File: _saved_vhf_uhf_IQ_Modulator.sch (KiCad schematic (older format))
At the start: 60 parts

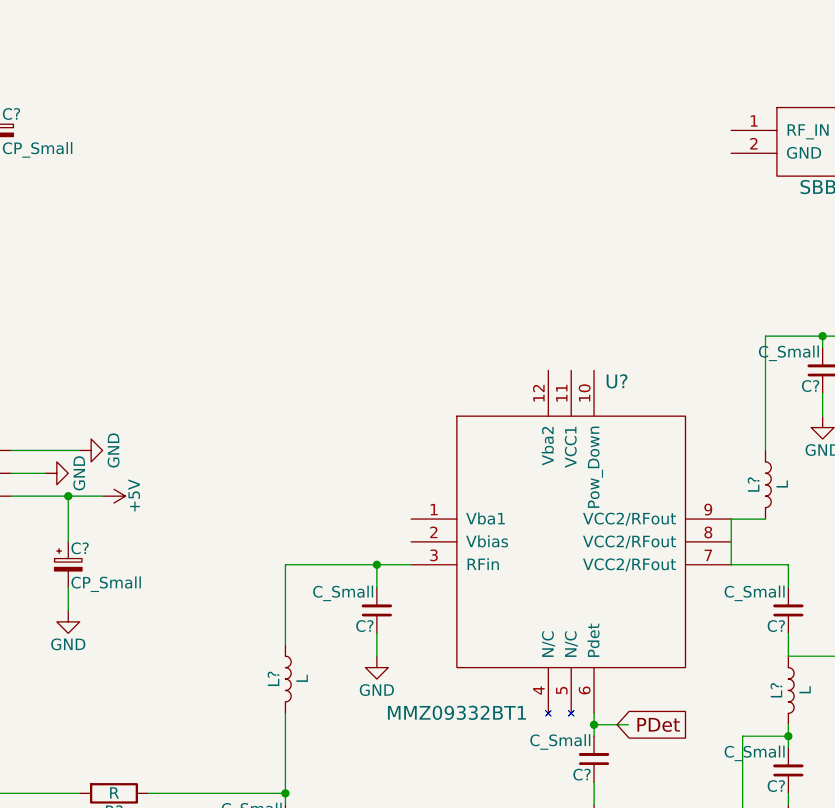
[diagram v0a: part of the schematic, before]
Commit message: added dokumets
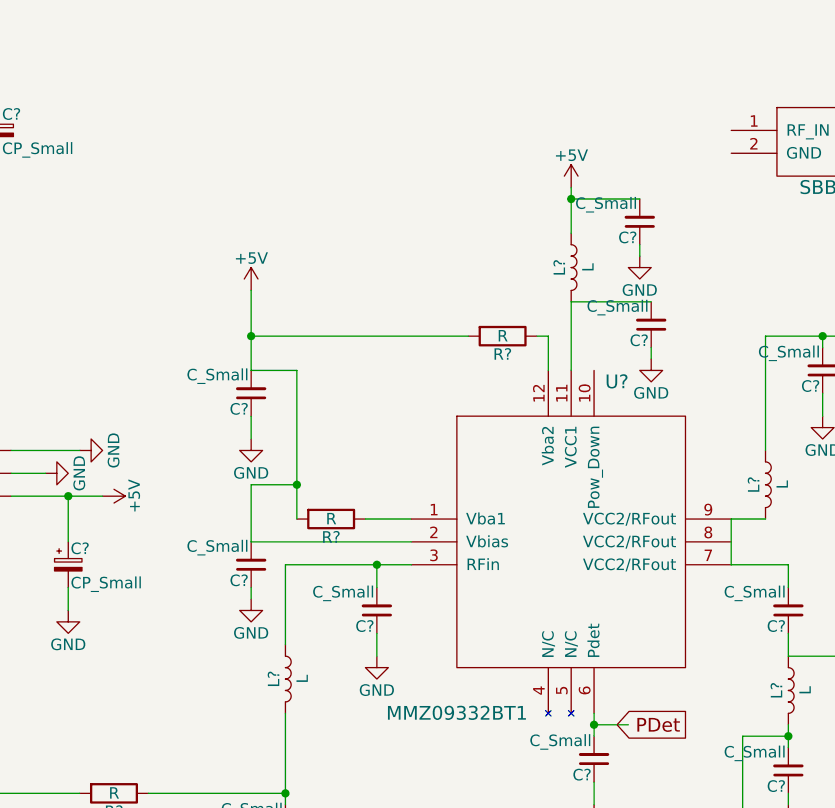
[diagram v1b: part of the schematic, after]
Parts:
- removed U?: MMZ09332BT1, symbol MMZ09332BT1
- added C? (x4): C_Small, symbol C_Small
- added L?: L, symbol L
- added R? (x2): R, symbol R
- added U?: MMZ09332BT1, symbol MMZ09332BT1
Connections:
- net +5V: now also C?.2, C?.2, C?.2, L?.1, R?.2, R?.2, U?.2 (Vbias)
- net GND: now also C?.1, C?.1, C?.1, C?.1
- net at C?.2, L?.1: now also U?.3 (RFin)
- net at C?.2: now also U?.6 (Pdet)
- net at C?.2, L?.2: now also U?.7 (VCC2/RFout), U?.9 (VCC2/RFout)
- new net: C?.2, L?.2, U?.11 (VCC1)
- new net: R?.1, U?.1 (Vba1)
- new net: R?.1, U?.12 (Vba2)
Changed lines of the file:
@@
-$EndComp
-$Comp
-L MMZ09332BT1 U?
-U 1 1 5A2315D3
-P 12850 3000
-F 0 "U?" H 13050 3700 60  0000 C CNN
-F 1 "MMZ09332BT1" H 12350 2250 60  0000 C CNN
-F 2 "" H 12850 3000 60  0001 C CNN
-F 3 "" H 12850 3000 60  0001 C CNN
-	1    12850 3000
-	1    0    0    -1
 $EndComp
 $Comp
@@
 	13100 3800 12950 3800
 Connection ~ 12950 3800
+$Comp
+L L L?
+U 1 1 5A2373B0
+P 12850 1800
+F 0 "L?" V 12800 1800 50  0000 C CNN
+F 1 "L" V 12925 1800 50  0000 C CNN
+F 2 "" H 12850 1800 50  0001 C CNN
+F 3 "" H 12850 1800 50  0001 C CNN
+	1    12850 1800
+	1    0    0    -1
+$EndComp
+$Comp
+L C_Small C?
+U 1 1 5A2374AB
+P 13200 2050
+F 0 "C?" H 13210 2120 50  0000 L CNN
+F 1 "C_Small" H 13210 1970 50  0000 L CNN
+F 2 "" H 13200 2050 50  0001 C CNN
+F 3 "" H 13200 2050 50  0001 C CNN
+	1    13200 2050
+	-1   0    0    1
+$EndComp
+$Comp
+L C_Small C?
+U 1 1 5A237595
+P 13150 1600
+F 0 "C?" H 13160 1670 50  0000 L CNN
+F 1 "C_Small" H 13160 1520 50  0000 L CNN
+F 2 "" H 13150 1600 50  0001 C CNN
+F 3 "" H 13150 1600 50  0001 C CNN
+	1    13150 1600
+	-1   0    0    1
+$EndComp
+Wire Wire Line
+	12850 2250 12850 1950
+Wire Wire Line
+	12850 1950 13200 1950
+$Comp
+L GND #PWR?
+U 1 1 5A237928
+P 13200 2200
+F 0 "#PWR?" H 13200 1950 50  0001 C CNN
+F 1 "GND" H 13200 2050 50  0000 C CNN
+F 2 "" H 13200 2200 50  0001 C CNN
+F 3 "" H 13200 2200 50  0001 C CNN
+	1    13200 2200
+	1    0    0    -1
+$EndComp
+$Comp
+L GND #PWR?
+U 1 1 5A237A2F
+P 13150 1750
+F 0 "#PWR?" H 13150 1500 50  0001 C CNN
+F 1 "GND" H 13150 1600 50  0000 C CNN
+F 2 "" H 13150 1750 50  0001 C CNN
+F 3 "" H 13150 1750 50  0001 C CNN
+	1    13150 1750
+	1    0    0    -1
+$EndComp
+$Comp
+L +5V #PWR?
+U 1 1 5A237AF7
+P 12850 1450
+F 0 "#PWR?" H 12850 1300 50  0001 C CNN
+F 1 "+5V" H 12850 1590 50  0000 C CNN
+F 2 "" H 12850 1450 50  0001 C CNN
+F 3 "" H 12850 1450 50  0001 C CNN
+	1    12850 1450
+	1    0    0    -1
+$EndComp
+Wire Wire Line
+	12850 1450 12850 1650
+Wire Wire Line
+	13150 1500 12850 1500
+Connection ~ 12850 1500
+Wire Wire Line
+	13150 1700 13150 1750
+Wire Wire Line
+	13200 2150 13200 2200
+$Comp
+L C_Small C?
+U 1 1 5A238059
+P 11450 3100
+F 0 "C?" H 11460 3170 50  0000 L CNN
+F 1 "C_Small" H 11460 3020 50  0000 L CNN
+F 2 "" H 11450 3100 50  0001 C CNN
+F 3 "" H 11450 3100 50  0001 C CNN
+	1    11450 3100
+	-1   0    0    1
+$EndComp
+$Comp
+L GND #PWR?
+U 1 1 5A23816D
+P 11450 3250
+F 0 "#PWR?" H 11450 3000 50  0001 C CNN
+F 1 "GND" H 11450 3100 50  0000 C CNN
+F 2 "" H 11450 3250 50  0001 C CNN
+F 3 "" H 11450 3250 50  0001 C CNN
+	1    11450 3250
+	1    0    0    -1
+$EndComp
+Wire Wire Line
+	11450 3200 11450 3250
+Wire Wire Line
+	11450 3000 12150 3000
+$Comp
+L R R?
+U 1 1 5A2384AF
+P 11800 2900
+F 0 "R?" V 11880 2900 50  0000 C CNN
+F 1 "R" V 11800 2900 50  0000 C CNN
+F 2 "" V 11730 2900 50  0001 C CNN
+F 3 "" H 11800 2900 50  0001 C CNN
+	1    11800 2900
+	0    1    1    0
+$EndComp
+$Comp
+L R R?
+U 1 1 5A2385C4
+P 12550 2100
+F 0 "R?" V 12630 2100 50  0000 C CNN
+F 1 "R" V 12550 2100 50  0000 C CNN
+F 2 "" V 12480 2100 50  0001 C CNN
+F 3 "" H 12550 2100 50  0001 C CNN
+	1    12550 2100
+	0    1    1    0
+$EndComp
+$Comp
+L C_Small C?
+U 1 1 5A2386CC
+P 11450 2350
+F 0 "C?" H 11460 2420 50  0000 L CNN
+F 1 "C_Small" H 11460 2270 50  0000 L CNN
+F 2 "" H 11450 2350 50  0001 C CNN
+F 3 "" H 11450 2350 50  0001 C CNN
+	1    11450 2350
+	-1   0    0    1
+$EndComp
+$Comp
+L GND #PWR?
+U 1 1 5A238803
+P 11450 2550
+F 0 "#PWR?" H 11450 2300 50  0001 C CNN
+F 1 "GND" H 11450 2400 50  0000 C CNN
+F 2 "" H 11450 2550 50  0001 C CNN
+F 3 "" H 11450 2550 50  0001 C CNN
+	1    11450 2550
+	1    0    0    -1
+$EndComp
+Wire Wire Line
+	11450 2450 11450 2550
+Wire Wire Line
+	11650 2900 11650 2250
+Wire Wire Line
+	11650 2250 11450 2250
+Wire Wire Line
+	11450 2250 11450 1900
+Wire Wire Line
+	12150 2900 11950 2900
+Wire Wire Line
+	12750 2250 12750 2100
+Wire Wire Line
+	12750 2100 12700 2100
+$Comp
+L +5V #PWR?
+U 1 1 5A239083
+P 11450 1900
+F 0 "#PWR?" H 11450 1750 50  0001 C CNN
+F 1 "+5V" H 11450 2040 50  0000 C CNN
+F 2 "" H 11450 1900 50  0001 C CNN
+F 3 "" H 11450 1900 50  0001 C CNN
+	1    11450 1900
+	1    0    0    -1
+$EndComp
+Wire Wire Line
+	11450 3000 11450 2750
+Wire Wire Line
+	11450 2750 11650 2750
+Connection ~ 11650 2750
+Wire Wire Line
+	12400 2100 11450 2100
+Connection ~ 11450 2100
+$Comp
+L MMZ09332BT1 U?
+U 1 1 5A239B90
+P 12850 3000
+F 0 "U?" H 13050 3700 60  0000 C CNN
+F 1 "MMZ09332BT1" H 12350 2250 60  0000 C CNN
+F 2 "" H 12850 3000 60  0001 C CNN
+F 3 "" H 12850 3000 60  0001 C CNN
+	1    12850 3000
+	1    0    0    -1
+$EndComp
 $EndSCHEMATC
